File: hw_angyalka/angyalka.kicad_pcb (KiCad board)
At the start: 2 copper layers, 82.9 x 59.5 mm, 34 parts, among them J1 Conn_2Rows-05Pins, Q1 AO3401A, Q2 AO3401A, SW1 SW_DPST_x2, T1 Tab, T2 Tab, T3 Tab, U1 PY32F002AF15P6TU

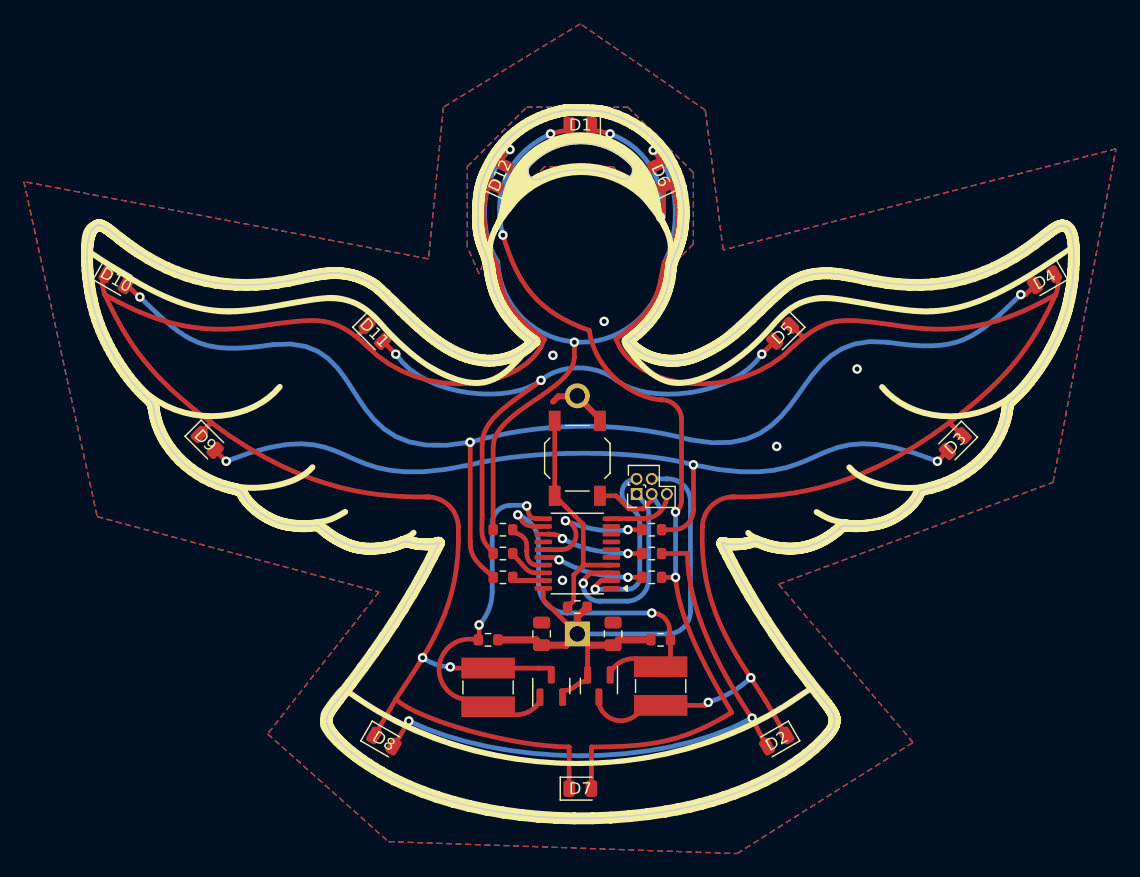
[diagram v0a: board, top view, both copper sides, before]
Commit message: Covered F.Mask around soldering pads
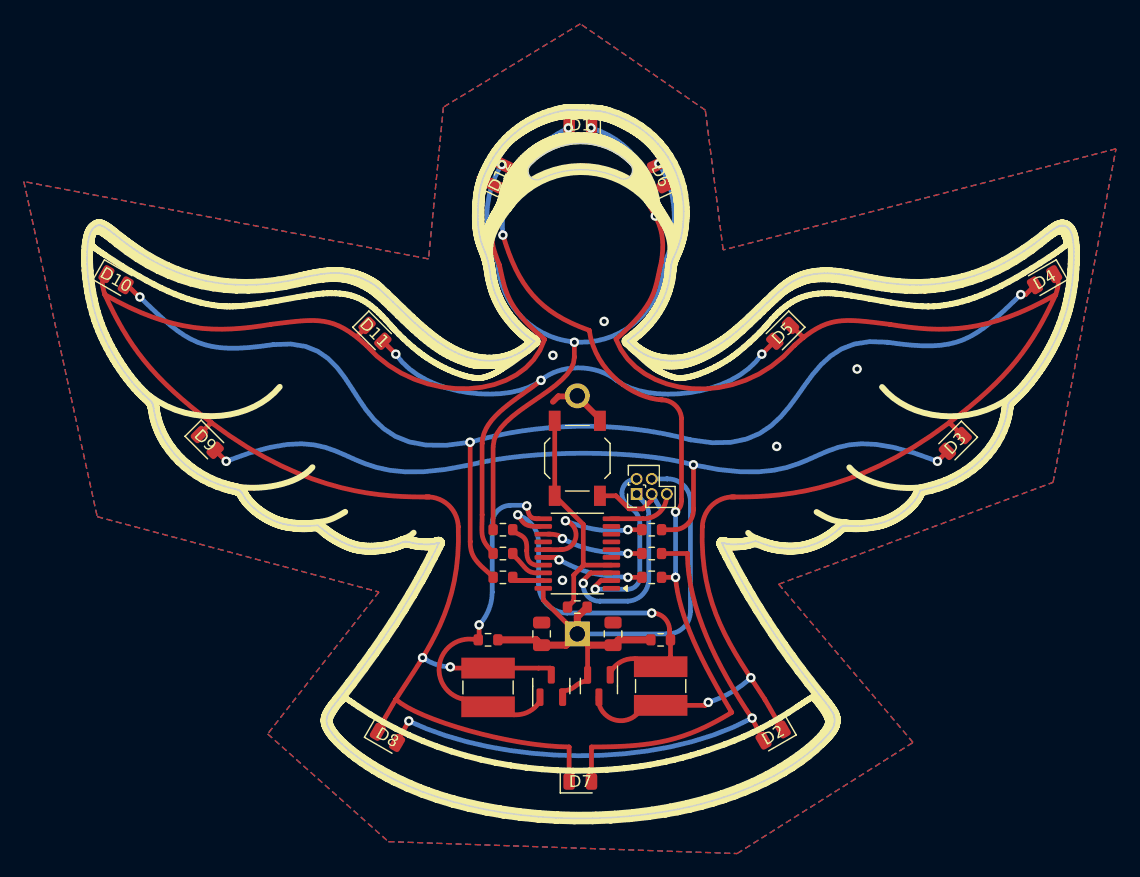
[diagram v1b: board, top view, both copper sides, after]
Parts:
- moved D7 0.60 mm to (148.5, 127.4)
- moved D2 0.58 mm to (164.7, 123.5)
- moved D8 0.42 mm to (132.3, 123.7)
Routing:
- net Net-(D1-K): track 8.21 -> 5.52 mm
- net Net-(D10-K): track 17.5 -> 16.9 mm
- net Net-(D1-A): track 17.0 -> 16.4 mm
- removed copper zone on B.Cu, net (none)
